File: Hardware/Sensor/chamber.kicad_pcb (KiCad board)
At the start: 2 copper layers, 83 x 95 mm, 42 parts, among them J1 Conn_01x15_Female, J2 Conn_01x15_Female, J3 RF_Shield_One_Piece, J4 Conn_Coaxial, J5 Conn_01x03_Male, J6 Conn_01x03_Male, U1 Nucleo32, U2 MCP3425A0T-ECH, U3 LMC662, U4 LM358

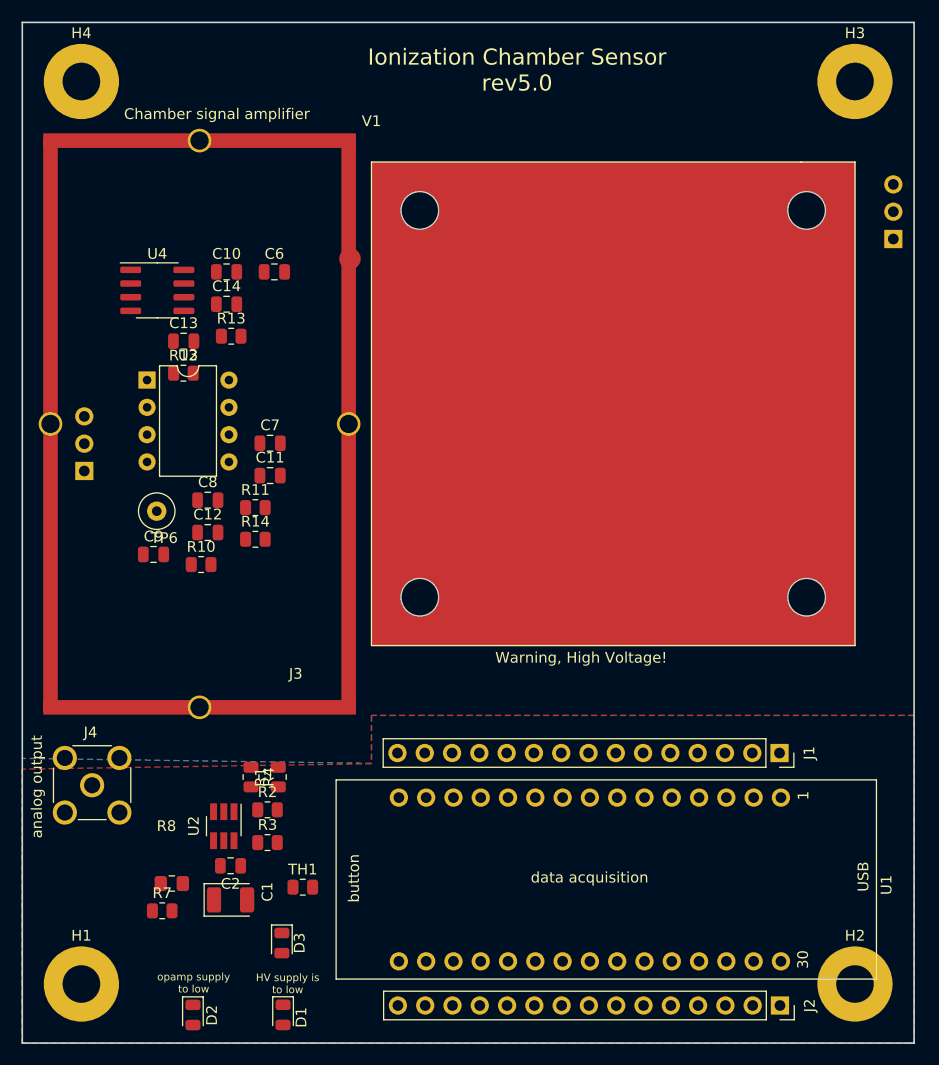
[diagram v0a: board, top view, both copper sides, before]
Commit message: draft of routing of sensor
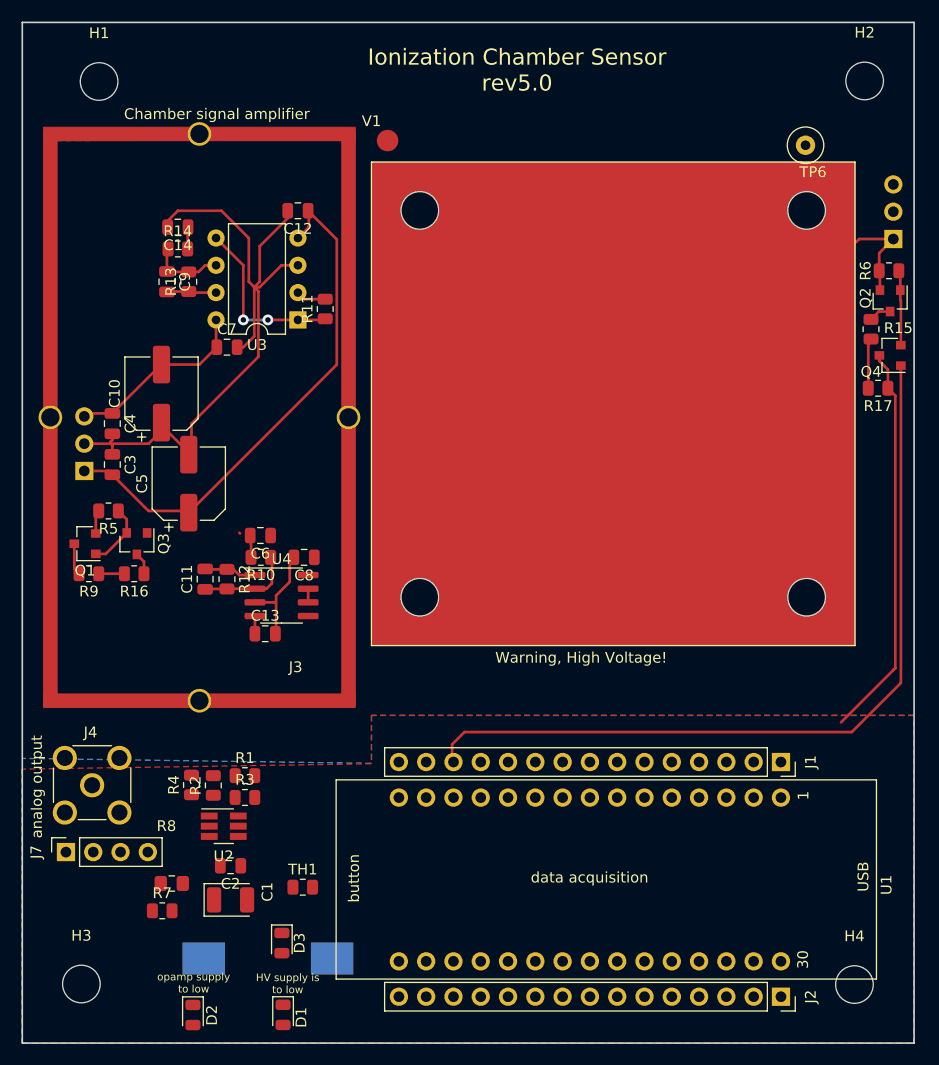
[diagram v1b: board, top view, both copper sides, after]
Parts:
- added BZ1: Buzzer, IonizationChamber:LPT1440S-HS-05-4.0-12-R, B.Cu at (79.9, 111.1)
- added C3: 100n, Capacitor_SMD:C_0805_2012Metric, F.Cu at (65.4, 65.2)
- added C4: 100n, Capacitor_SMD:C_0805_2012Metric, F.Cu at (65.4, 61.3)
- added C5: CP, Capacitor_SMD:CP_Elec_6.3x5.8, F.Cu at (72.5, 66.9)
- added J7: Conn_01x04_Female, Connector_PinSocket_2.54mm:PinSocket_1x04_P2.54mm_Vertical, F.Cu at (61.1, 101.2)
- added Q1: Q_PMOS_GDS, Package_TO_SOT_SMD:SOT-23, F.Cu at (62.8, 72.5)
- added Q2: Q_PMOS_GDS, Package_TO_SOT_SMD:SOT-23, F.Cu at (137.8, 49.9)
- added Q3: Q_NMOS_GDS, Package_TO_SOT_SMD:SOT-23, F.Cu at (67.7, 72.5)
- added Q4: Q_NMOS_GDS, Package_TO_SOT_SMD:SOT-23, F.Cu at (137.8, 55.0)
- added R15: TBD, Resistor_SMD:R_0805_2012Metric, F.Cu at (136.0, 52.6)
- added R16: TBD, Resistor_SMD:R_0805_2012Metric, F.Cu at (67.4, 75.3)
- added R17: TBD, Resistor_SMD:R_0805_2012Metric, F.Cu at (136.7, 58.0)
- added R5: TBD, Resistor_SMD:R_0805_2012Metric, F.Cu at (65.0, 69.5)
- added R6: TBD, Resistor_SMD:R_0805_2012Metric, F.Cu at (137.7, 47.1)
- added R9: TBD, Resistor_SMD:R_0805_2012Metric, F.Cu at (63.2, 75.3)
- C10: value not mounted -> CP; footprint Capacitor_SMD:C_0805_2012Metric -> Capacitor_SMD:CP_Elec_6.3x5.8
- D1: value yellow -> red
- H1, H2, H3, H4: value MountingHole_Pad -> MountingHole; footprint MountingHole:MountingHole_3.5mm_Pad -> MountingHole:MountingHole_3.5mm
- moved H4 110.6 mm to (134.4, 113.5)
- moved H3 110.6 mm to (62.5, 113.5)
- moved H2 84.1 mm to (135.4, 29.4)
- moved H1 84.0 mm to (64.2, 29.5)
- moved TP6 69.3 mm to (129.9, 35.4)
- moved C12 31.1 mm to (82.7, 41.5), turned to 180 degrees
- moved U4 30.7 mm to (81.1, 77.3)
- moved C13 28.3 mm to (79.6, 80.9)
- moved R14 28.0 mm to (71.5, 45.1)
- moved C9 25.4 mm to (70.5, 48.1), turned to 270 degrees
- moved C6 24.6 mm to (79.2, 71.8), turned to 180 degrees
- moved R11 19.6 mm to (85.2, 50.7), turned to 90 degrees
- moved R12 19.6 mm to (76.0, 75.8), turned to 270 degrees
- moved U3 15.1 mm to (82.7, 51.7), turned to 180 degrees
- moved C10 12.8 mm to (70.0, 58.5), turned to 90 degrees
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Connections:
- net Net-(J1-Pad10) renamed BATTERY_MEASSURE_ENA
- net Net-(J1-Pad11) renamed BATTERY_MEASSURE_VALUE
- net Net-(J1-Pad12) renamed CHAMBER_VOLTAGE_MEASSURE_VALUE
- net Net-(J1-Pad13) renamed CHAMBER_VOLTAGE_MEASSURE_ENA
- C10 pad 1: Net-(C10-Pad1) -> GND
- C10 pad 2: Net-(C10-Pad2) -> +BATT
- H1 pad 1: GND -> (no net)
- H2 pad 1: GND -> (no net)
- H3 pad 1: GND -> (no net)
- H4 pad 1: GND -> (no net)
- J5 pad 1: (no net) -> /AnalogFrontend/CHAMBER_VOLTAGE
- J6 pad 1: (no net) -> -BATT
- J6 pad 2: (no net) -> GND
- J6 pad 3: (no net) -> +BATT
- R11 pad 1: Net-(C10-Pad1) -> Net-(R11-Pad1)
- R11 pad 2: Net-(C10-Pad2) -> Net-(R11-Pad2)
- TP6 pad 1: +BATT -> /AnalogFrontend/CHAMBER_VOLTAGE
- U3 pad 1: Net-(C10-Pad1) -> Net-(R11-Pad1)
- U3 pad 2: Net-(C10-Pad2) -> Net-(R11-Pad2)
- U3 pad 5: Net-(C10-Pad1) -> Net-(R11-Pad1)
- V1 pad 1: +BATT -> /AnalogFrontend/CHAMBER_VOLTAGE
- V1 pad 2: Net-(C10-Pad2) -> Net-(R11-Pad2)
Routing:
- net GND: track 0.00 -> 116.0 mm
- net CHAMBER_VOLTAGE_MEASSURE_ENA: track 0.00 -> 74.5 mm
- net -BATT: track 0.00 -> 50.9 mm
- net /AnalogFrontend/CHAMBER_VOLTAGE: track 0.00 -> 24.3 mm
- net +BATT: track 0.00 -> 19.8 mm
- net Net-(R11-Pad1): track 0.00 -> 16.3 mm, vias 0 -> 2
- net Net-(C11-Pad1): track 0.00 -> 8.87 mm
- net Net-(Q2-Pad1): track 0.00 -> 7.00 mm
- net Net-(C9-Pad1): track 0.00 -> 6.98 mm
- net Net-(Q1-Pad1): track 0.00 -> 6.06 mm
- net CHAMBER_VOLTAGE_MEASSURE_VALUE: track 0.00 -> 5.18 mm
- net Net-(C11-Pad2): track 0.00 -> 4.82 mm
- net Net-(C6-Pad1): track 0.00 -> 4.63 mm
- net Net-(Q1-Pad3): track 0.00 -> 2.98 mm
- net Net-(R11-Pad2): track 0.00 -> 2.79 mm
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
